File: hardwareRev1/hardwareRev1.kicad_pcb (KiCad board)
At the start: 2 copper layers, 60 parts, among them J1 MicroSD, J2 SMA, K1 PWMOut, K2 ADC1, P1 UART, P10 ID, P2 I2C, P3 ADC2, P4 CONN_7, P5 CONN_5X2, P6 CONN_11X2, P7 GPSDM, P8 GPSDP, Q1 MOS_P_NUM, U1 MKL26Z128VLH4, U2 24C16, U3 MICRO-B_USB, X1 CRYSTAL_ABM3C

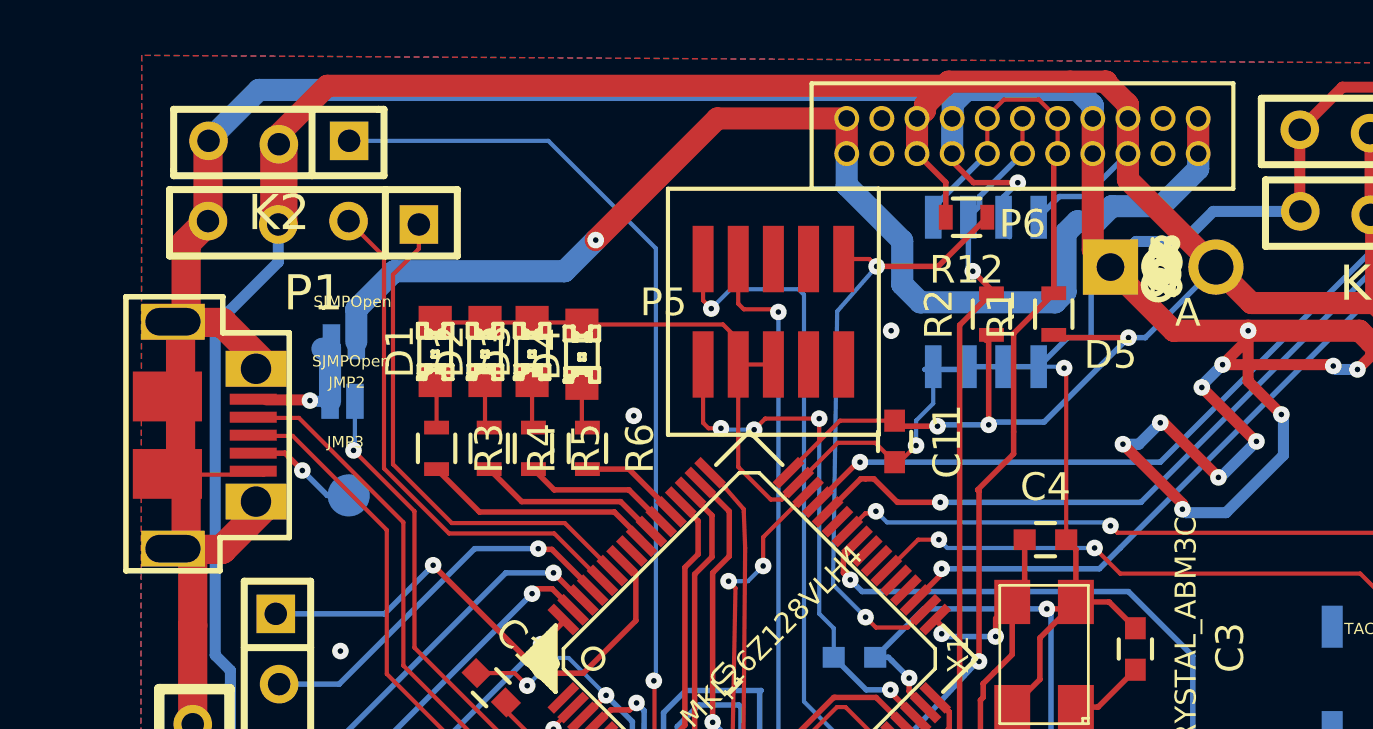
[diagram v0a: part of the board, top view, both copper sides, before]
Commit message: added the radio .
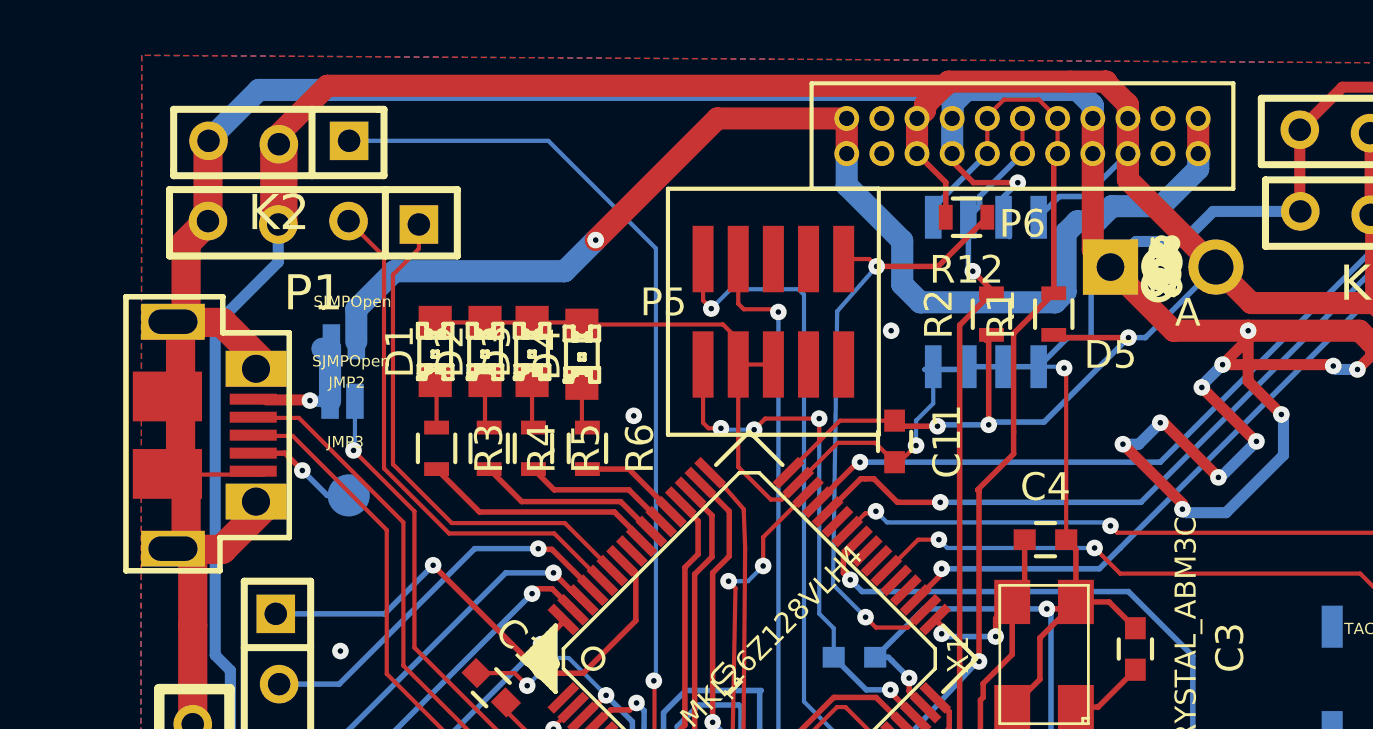
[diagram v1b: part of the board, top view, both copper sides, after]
